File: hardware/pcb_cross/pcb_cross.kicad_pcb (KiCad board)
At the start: 2 copper layers, 99.7 x 87 mm, 11 parts, among them J1 C96ABC, J2 C96ABC, J3 C96ABC, J4 C96ABC, J5 C96ABC, J6 PWR1, J7 PWR2

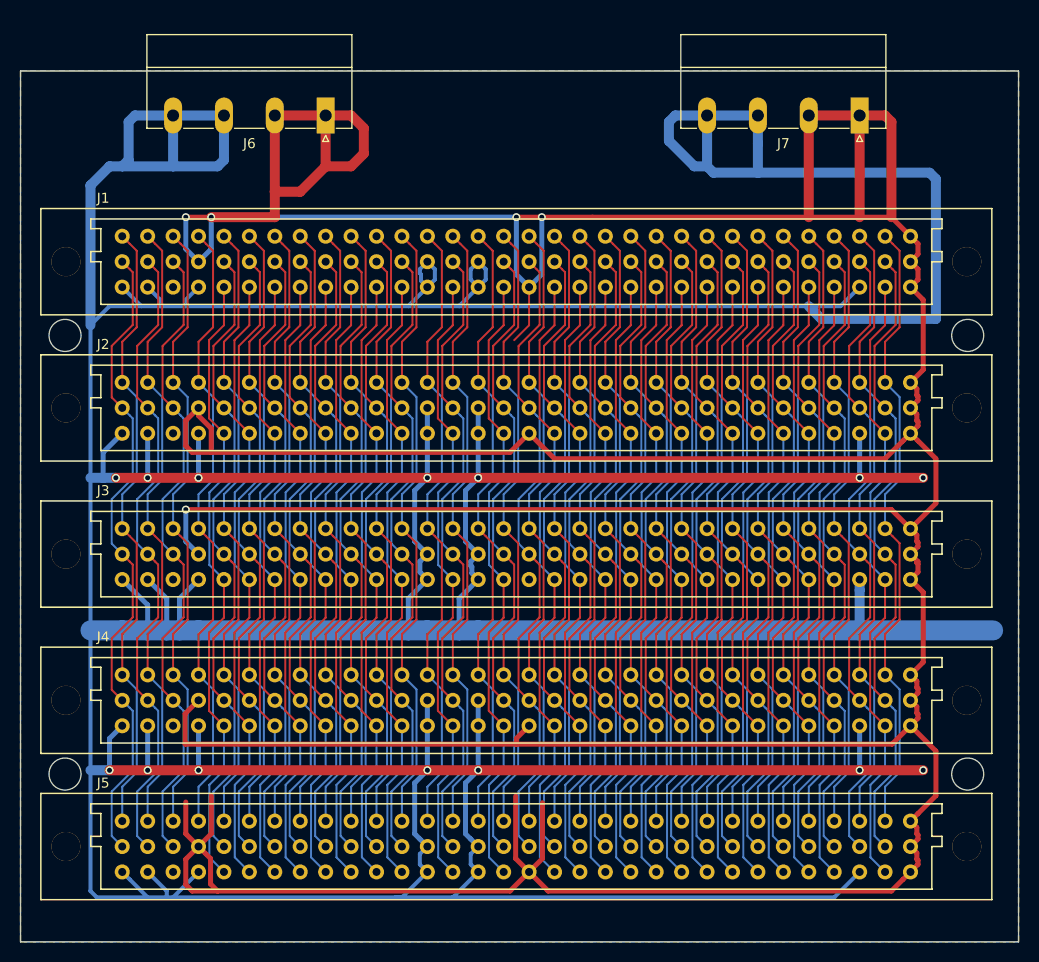
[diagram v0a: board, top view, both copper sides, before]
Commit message: Актуализированна аппаратная часть
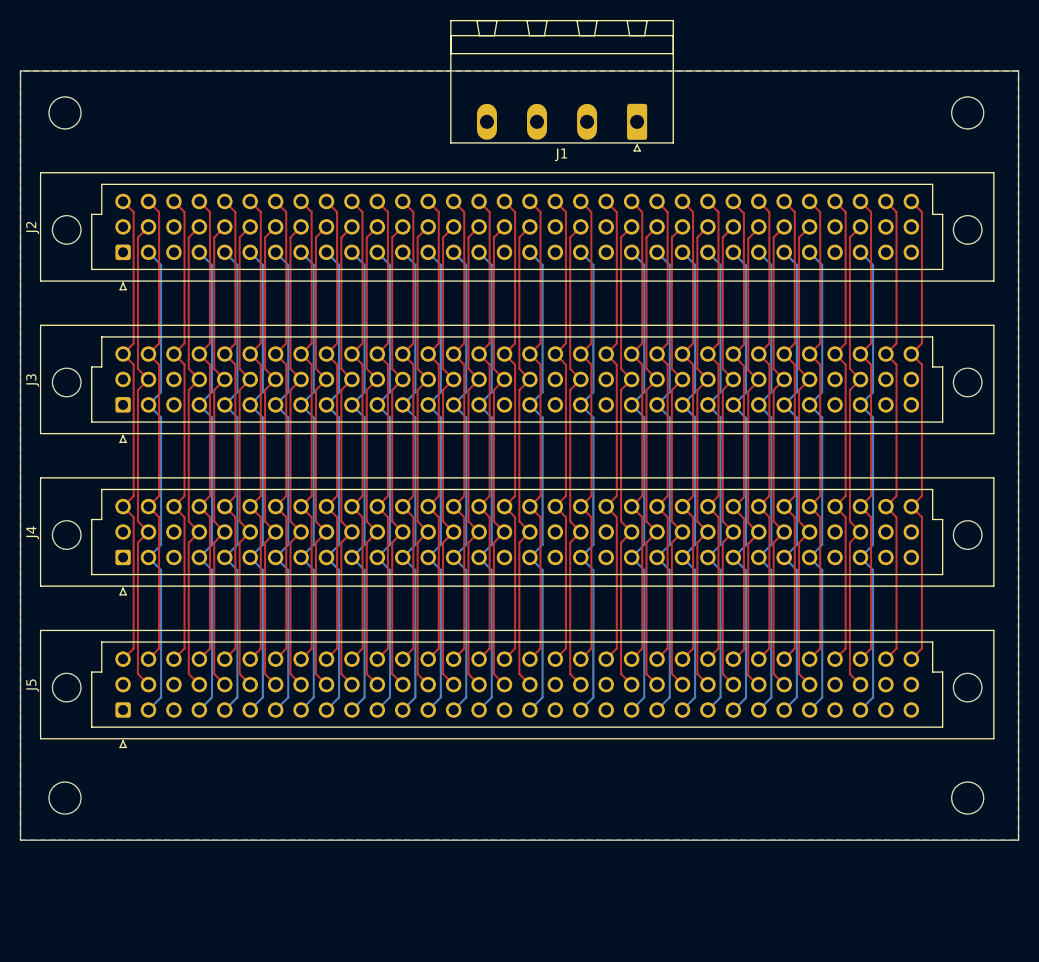
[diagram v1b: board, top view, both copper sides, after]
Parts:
- removed J6: PWR1, Connectors_Phoenix:PhoenixContact_MC-G_04x5.08mm_Angled
- removed J7: PWR2, Connectors_Phoenix:PhoenixContact_MC-G_04x5.08mm_Angled
- J1: value C96ABC -> Screw_Terminal_01x04; footprint orion:Socket_DIN41612-CaseC1-full-Female-96Pin-3rows -> Connector_Phoenix_MSTB:PhoenixContact_MSTBA_2,5_4-G_1x04_P5.00mm_Horizontal
- J2, J3, J4, J5: footprint orion:Socket_DIN41612-CaseC1-full-Female-96Pin-3rows -> Connector_DIN:DIN41612_C_3x32_Female_Vertical_THT
- moved J2 42.2 mm to (109.9, 81.6), turned to 90 degrees
- moved J3 42.0 mm to (109.9, 96.9), turned to 90 degrees
- moved J4 41.8 mm to (109.9, 112.1), turned to 90 degrees
- moved J5 41.6 mm to (109.9, 127.3), turned to 90 degrees
- moved REF** 22.2 mm to (194.3, 67.7)
- moved REF** 22.2 mm to (104.1, 67.7)
- moved J1 18.5 mm to (161.3, 68.6), turned to 180 degrees
- moved REF** 2.40 mm to (104.1, 136.1)
- moved REF** 2.40 mm to (194.3, 136.1)
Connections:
- J1 pad 1: (no net) -> VCC
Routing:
- net VCC: track 793.9 -> 0.00 mm, vias 14 -> 0
- net GND: track 616.8 -> 48.3 mm, vias 5 -> 0
- net /7B: track 65.4 -> 0.00 mm
- net /3B: track 65.4 -> 0.00 mm
- net /26B: track 65.4 -> 0.00 mm
- net /25B: track 65.4 -> 0.00 mm
- net /21B: track 65.4 -> 0.00 mm
- net /14B: track 65.4 -> 0.00 mm
- net /9B: track 65.4 -> 0.00 mm
- net /6B: track 65.4 -> 0.00 mm
- net /2B: track 65.4 -> 0.00 mm
- net /24B: track 65.4 -> 0.00 mm
- net /17B: track 65.4 -> 0.00 mm
- net /13B: track 65.4 -> 0.00 mm
- net /10B: track 65.4 -> 0.00 mm
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- added copper zone on B.Cu, net GND
- added copper zone on In1.Cu, net GND
- added copper zone on In2.Cu, net VCC
- removed copper zone on B.Cu, net VCC
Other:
- board size 99.7 x 87 mm -> 99.7 x 76.8 mm
- copper layers 2 -> 4
- net class Default removed
